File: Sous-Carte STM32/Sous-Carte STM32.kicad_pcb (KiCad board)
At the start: 2 copper layers, 113 x 120.1 mm, 34 parts, among them J1 RJ45, P1 CONN_25X2, P2 CONN_25X2, P3 CONN_4, P5 CONN_25X2, P6 CONN_2, P7 CONN_2, P8 CONN_2

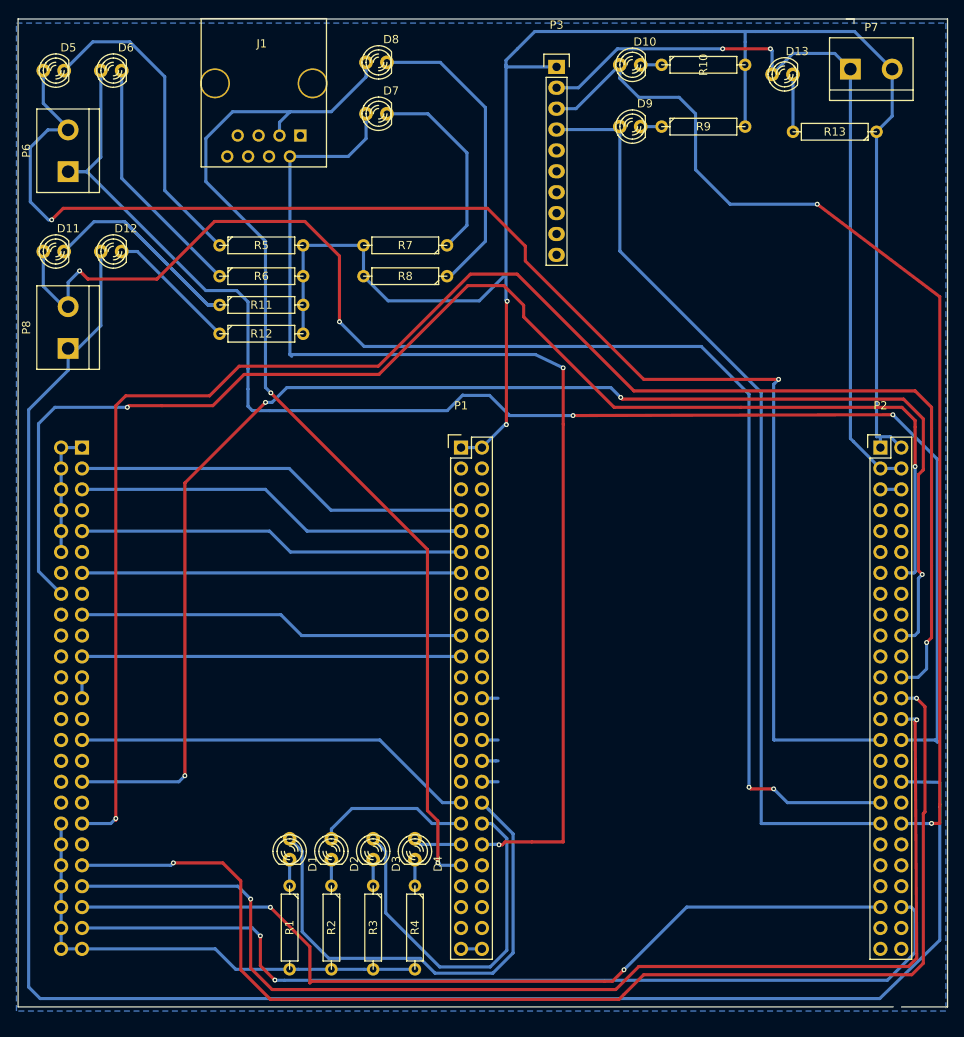
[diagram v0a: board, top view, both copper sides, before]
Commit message: plus que 3 piste a router 2 ou trois truc a revoir
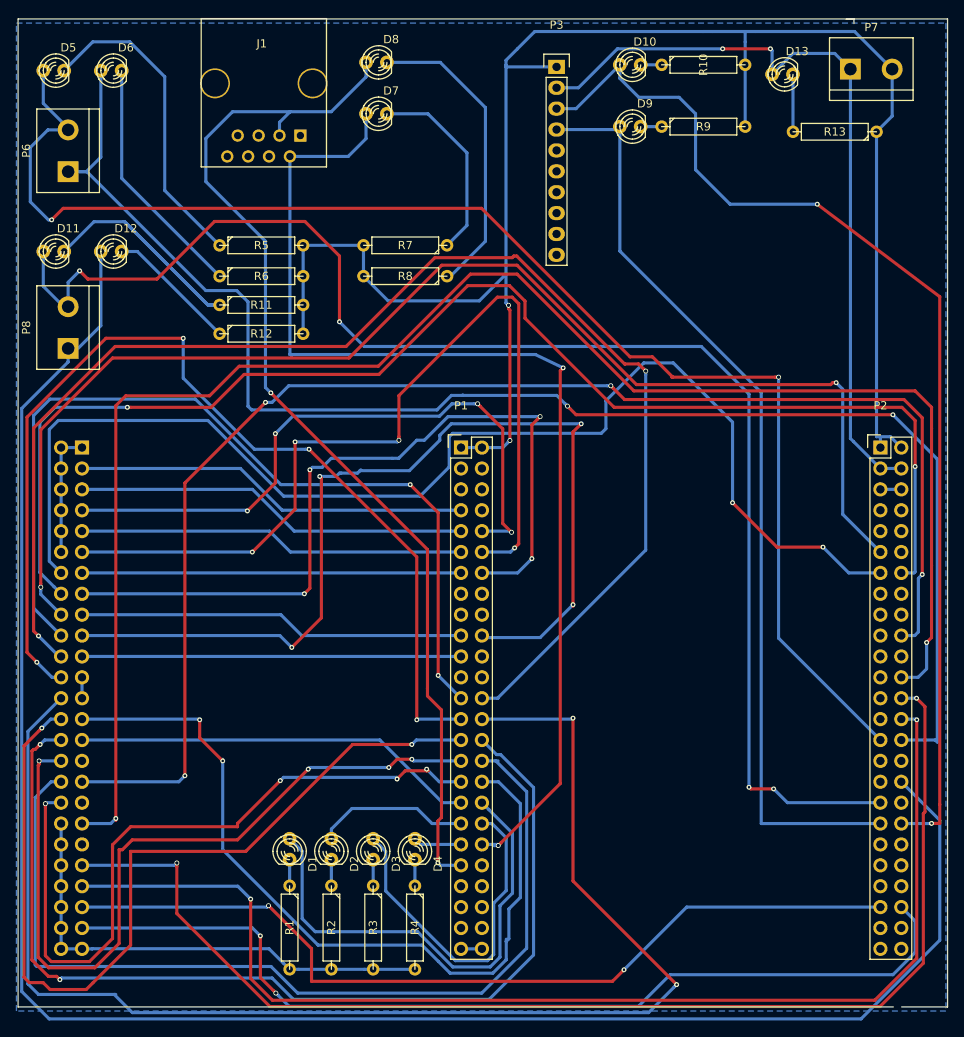
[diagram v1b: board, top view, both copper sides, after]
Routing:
- net E10: track 0.00 -> 167.1 mm, vias 0 -> 2
- net E8: track 1.96 -> 167.5 mm, vias 0 -> 2
- net E6: track 0.00 -> 157.5 mm, vias 0 -> 2
- net E4: track 0.00 -> 150.5 mm, vias 0 -> 2
- net E9: track 0.00 -> 124.6 mm, vias 0 -> 4
- net E12: track 1.96 -> 123.9 mm, vias 0 -> 2
- net C4: track 0.00 -> 118.9 mm, vias 0 -> 4
- net E14: track 1.96 -> 114.0 mm
- net A0: track 0.00 -> 108.5 mm, vias 0 -> 4
- net E7: track 0.00 -> 107.6 mm, vias 0 -> 2
- net E11: track 0.00 -> 107.0 mm, vias 0 -> 2
- net A2: track 0.00 -> 97.7 mm, vias 0 -> 4
- net B10: track 1.96 -> 98.6 mm, vias 0 -> 2
- net E13: track 0.00 -> 95.8 mm, vias 0 -> 4
- net E15: track 0.00 -> 89.3 mm, vias 0 -> 4
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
